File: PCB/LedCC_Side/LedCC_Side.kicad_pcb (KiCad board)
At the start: 2 copper layers, 84.5 x 19.7 mm, 19 parts, among them J1 In, J2 Out, J3 In, J4 Out

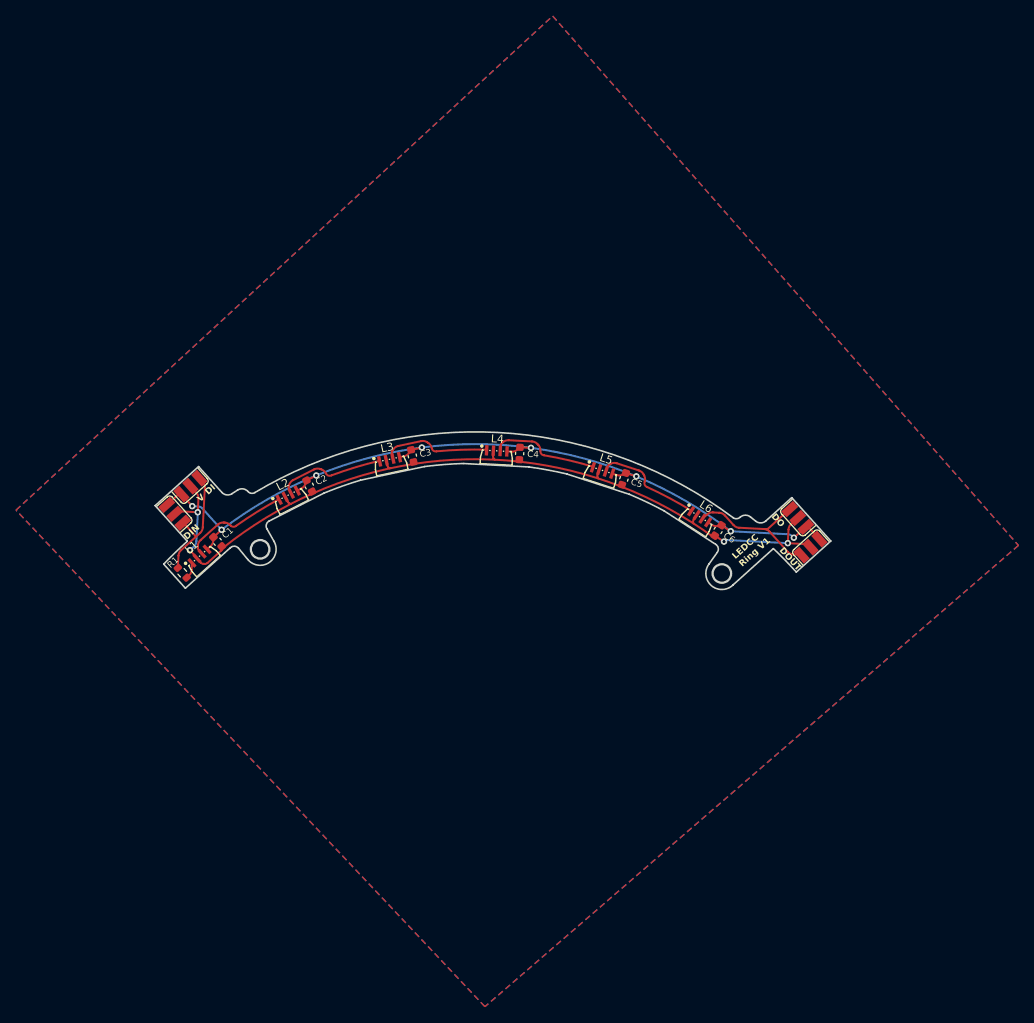
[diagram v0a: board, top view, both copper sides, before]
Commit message: PCB Updates
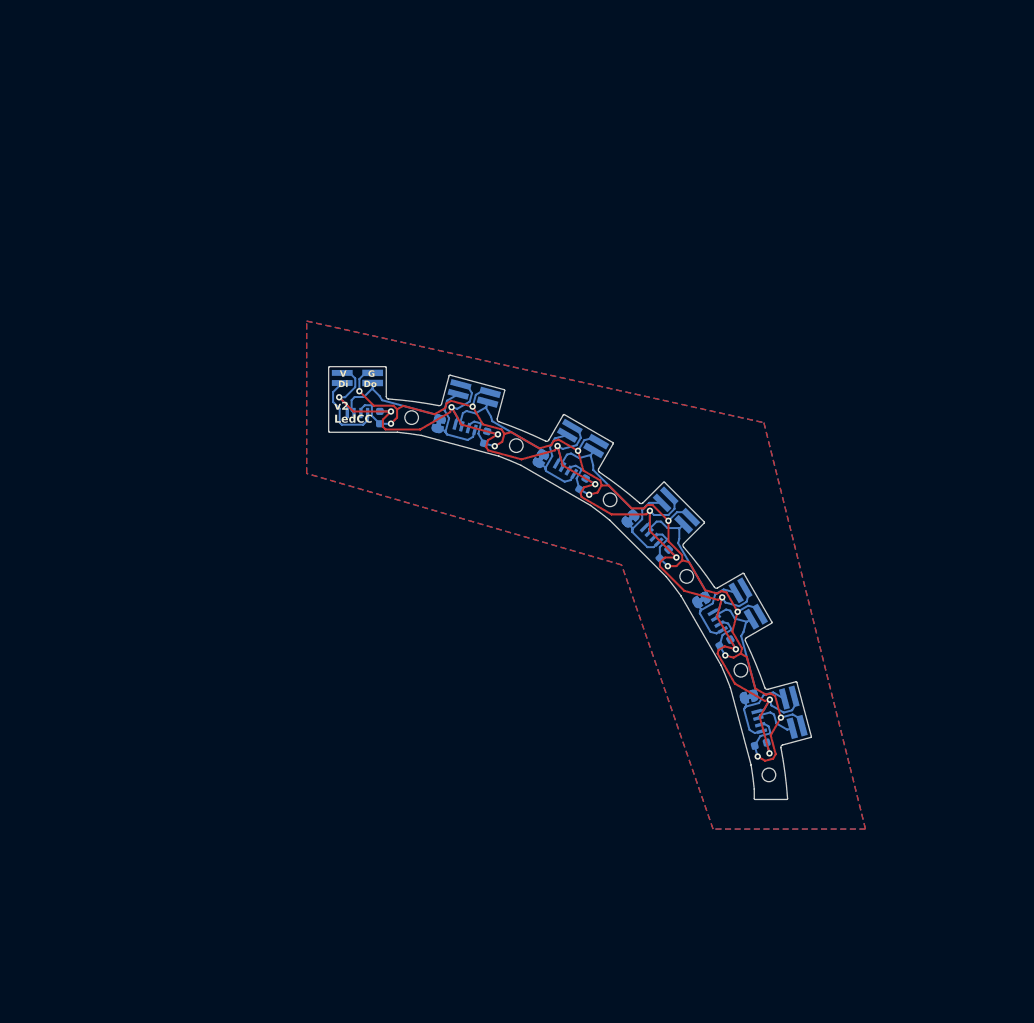
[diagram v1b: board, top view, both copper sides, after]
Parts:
- removed H1, H2: MountingHole, MountingHole:MountingHole_2.2mm_M2
- removed R1: 330, Resistor_SMD:R_0603_1608Metric
- added J5: Conn_01x04, Library:HDR-SMD_4P-P1.27-V-M-R2-C2-S1.27-LS5.5, B.Cu at (198.8, 71.8)
- added J6: Conn_01x04, Library:HDR-SMD_4P-P1.27-V-M-R2-C2-S1.27-LS5.5, B.Cu at (204.5, 85.4)
- added JP2: Jumper_2_Small_Bridged, Jumper:SolderJumper-2_P1.3mm_Bridged_RoundedPad1.0x1.5mm, B.Cu at (160.2, 49.3)
- added JP3: Jumper_2_Small_Bridged, Jumper:SolderJumper-2_P1.3mm_Bridged_RoundedPad1.0x1.5mm, B.Cu at (172.9, 53.7)
- added JP4: Jumper_2_Small_Bridged, Jumper:SolderJumper-2_P1.3mm_Bridged_RoundedPad1.0x1.5mm, B.Cu at (184.1, 61.2)
- added JP5: Jumper_2_Small_Bridged, Jumper:SolderJumper-2_P1.3mm_Bridged_RoundedPad1.0x1.5mm, B.Cu at (193.0, 71.4)
- added JP6: Jumper_2_Small_Bridged, Jumper:SolderJumper-2_P1.3mm_Bridged_RoundedPad1.0x1.5mm, B.Cu at (199.0, 83.5)
- C1, C2, C3, C4, C5, C6, L1, L2, L3, L4, L5, L6: moved to B.Cu
- J1, J3: value In -> Conn_01x04; footprint Library:Led-Jumper -> Library:HDR-SMD_4P-P1.27-V-M-R2-C2-S1.27-LS5.5; moved to B.Cu
- J2, J4: value Out -> Conn_01x04; footprint Library:Led-Jumper -> Library:HDR-SMD_4P-P1.27-V-M-R2-C2-S1.27-LS5.5; moved to B.Cu
- moved J3 49.4 mm to (178.2, 51.2), turned to 60 degrees
- moved J2 46.1 mm to (164.6, 45.5), turned to 75 degrees
- moved J1 28.3 mm to (150.0, 43.6), turned to 90 degrees
- moved C6 27.2 mm to (200.4, 89.4), turned to 15 degrees
- moved L6 26.6 mm to (200.2, 86.5), turned to -75 degrees
- moved L1 26.6 mm to (150.0, 48.0), turned to 0 degrees
- moved C1 25.5 mm to (152.8, 48.6), turned to 90 degrees
- moved C5 24.1 mm to (195.9, 76.7), turned to 30 degrees
- moved L5 23.7 mm to (195.0, 74.0), turned to -60 degrees
- moved L2 23.7 mm to (163.5, 49.8), turned to -15 degrees
- moved C2 22.9 mm to (166.0, 51.0), turned to 75 degrees
- moved L4 22.0 mm to (186.8, 63.2), turned to -45 degrees
- moved L3 22.0 mm to (176.0, 55.0), turned to -30 degrees
- moved C4 22.0 mm to (188.3, 65.6), turned to 45 degrees
- moved C3 21.6 mm to (178.1, 56.9), turned to 60 degrees
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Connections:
- J1 pad 1: GND -> /Din
- J1 pad 2: VDD -> /Dout
- J1 pad 3: DIN -> GND
- J2 pad 1: GND -> Net-(J2-Pin_1)
- J2 pad 2: VDD -> Net-(J2-Pin_2)
- J2 pad 3: DOUT -> GND
- J3 pad 1: GND -> Net-(J3-Pin_1)
- J3 pad 2: VDD -> Net-(J3-Pin_2)
- J3 pad 3: DIN -> GND
- J4 pad 1: GND -> Net-(J4-Pin_1)
- J4 pad 2: VDD -> Net-(J4-Pin_2)
- J4 pad 3: DOUT -> GND
- L1 pad 1: Net-(L1-DIN) -> /Din
- L1 pad 3: Net-(L1-DOUT) -> /Dout
- L2 pad 1: Net-(L1-DOUT) -> Net-(J2-Pin_1)
- L2 pad 3: Net-(L2-DOUT) -> Net-(J2-Pin_2)
- L3 pad 1: Net-(L2-DOUT) -> Net-(J3-Pin_1)
- L3 pad 3: Net-(L3-DOUT) -> Net-(J3-Pin_2)
- L4 pad 1: Net-(L3-DOUT) -> Net-(J4-Pin_1)
- L4 pad 3: Net-(L4-DOUT) -> Net-(J4-Pin_2)
- L5 pad 1: Net-(L4-DOUT) -> Net-(J5-Pin_1)
- L5 pad 3: Net-(L5-DOUT) -> Net-(J5-Pin_2)
- L6 pad 1: Net-(L5-DOUT) -> Net-(J6-Pin_1)
- L6 pad 3: DOUT -> Net-(J6-Pin_2)
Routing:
- net GND: track 105.5 -> 154.2 mm, vias 8 -> 12
- net VDD: track 104.1 -> 149.0 mm, vias 4 -> 12
- net DOUT: track 18.7 -> 0.00 mm
- net Net-(J3-Pin_2): track 0.00 -> 14.9 mm
- net Net-(J5-Pin_2): track 0.00 -> 14.9 mm
- net Net-(J4-Pin_2): track 0.00 -> 14.9 mm
- net /Dout: track 0.00 -> 14.9 mm
- net Net-(J2-Pin_2): track 0.00 -> 14.9 mm
- net DIN: track 14.4 -> 0.00 mm
- net Net-(L1-DOUT): track 13.7 -> 0.00 mm
- net Net-(L5-DOUT): track 13.7 -> 0.00 mm
- net Net-(L3-DOUT): track 13.7 -> 0.00 mm
- net Net-(L2-DOUT): track 13.7 -> 0.00 mm
- net Net-(L4-DOUT): track 13.7 -> 0.00 mm
- net Net-(J5-Pin_1): track 0.00 -> 12.0 mm
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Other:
- board size 84.5 x 19.7 mm -> 60.3 x 54.1 mm
- board text added: "V G Di Do"
- board text added: "v2 LedCC"
- board text removed: "DI"
- board text removed: "DIN"
- board text removed: "DO"
- board text removed: "DOUT"
- board text removed: "LEDCC Ring V1"
- board text removed: "V"
